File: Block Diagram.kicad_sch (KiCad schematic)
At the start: 0 parts

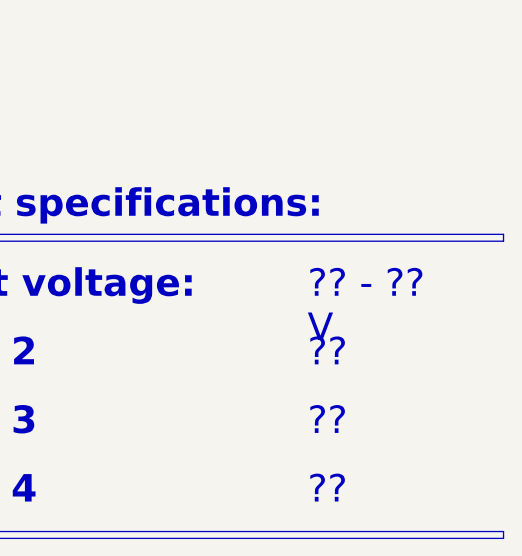
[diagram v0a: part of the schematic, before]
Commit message: chore: Update project file names and paths for Linux-Kit
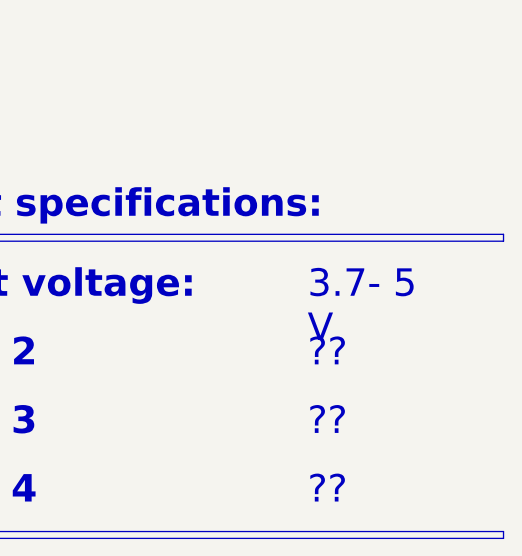
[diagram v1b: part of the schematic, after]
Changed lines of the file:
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@@
 		)
 	)
-	(text_box "?? - ?? V"
+	(text_box "3.7- 5 V"
 		(exclude_from_sim no)
 		(at 378.46 205.74 0)
